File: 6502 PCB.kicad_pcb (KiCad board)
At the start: 2 copper layers, 99.1 x 83.8 mm, 21 parts, among them J1 power_source, J17 Conn_01x16_Pin, J2 Conn_01x02_Pin, SW1 RESET, U1 W65C02S, U2 28C256, U3 62256, U4 W65C22, U5 74HC00, X1 1MHz

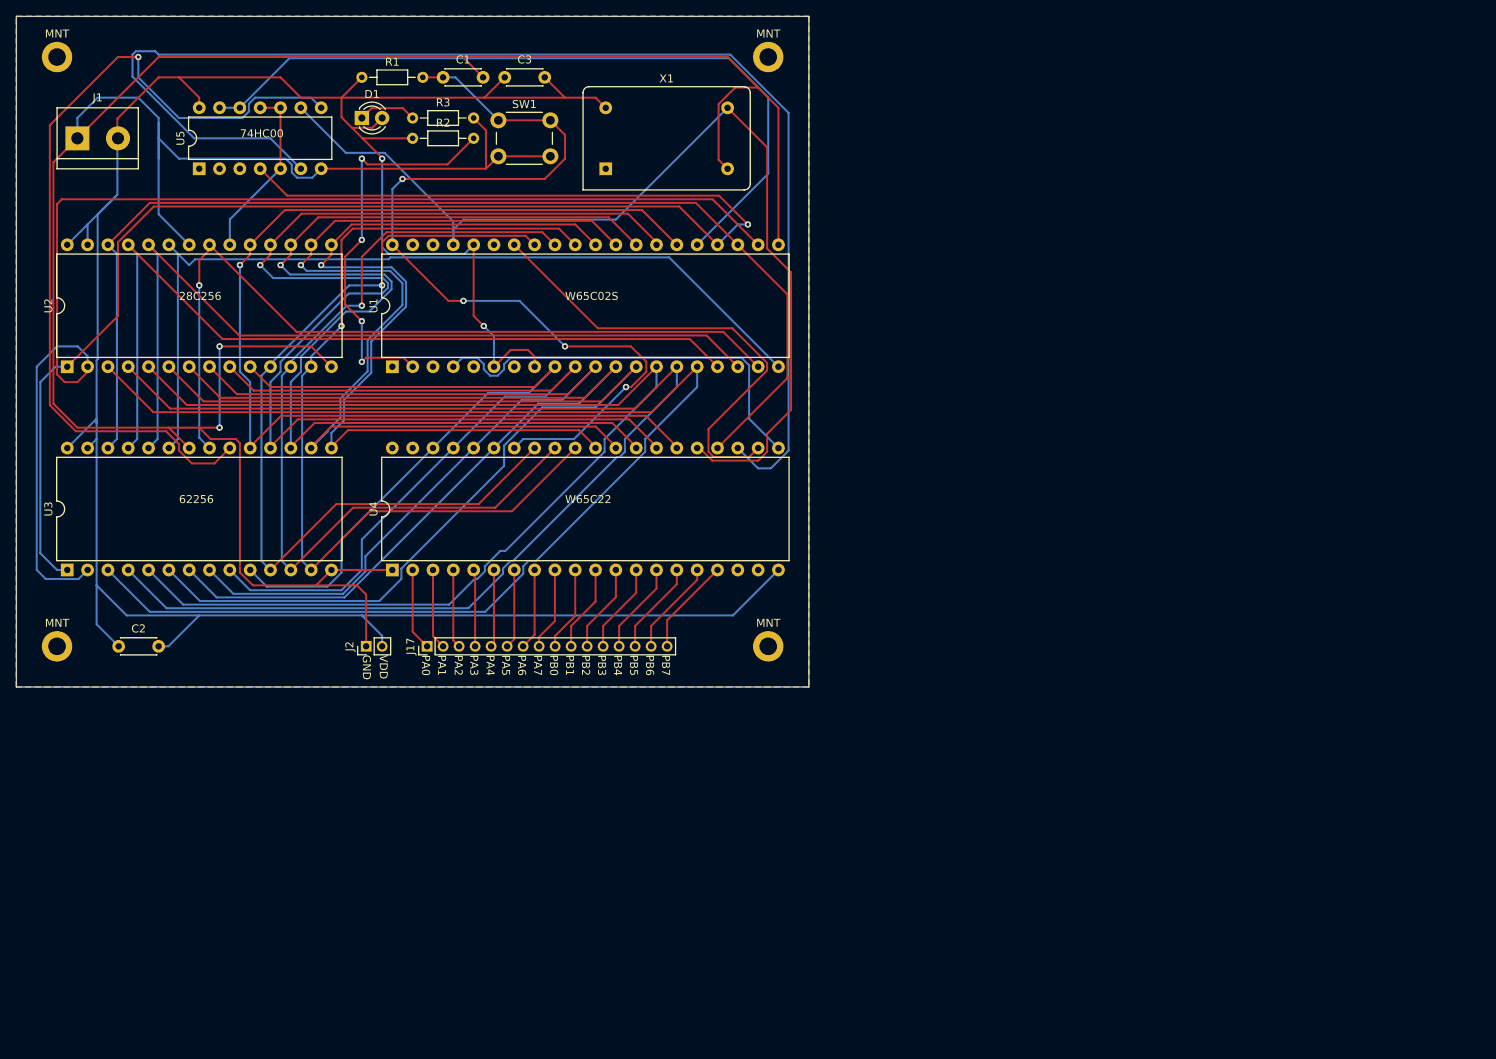
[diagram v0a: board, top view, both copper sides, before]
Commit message: aaaa
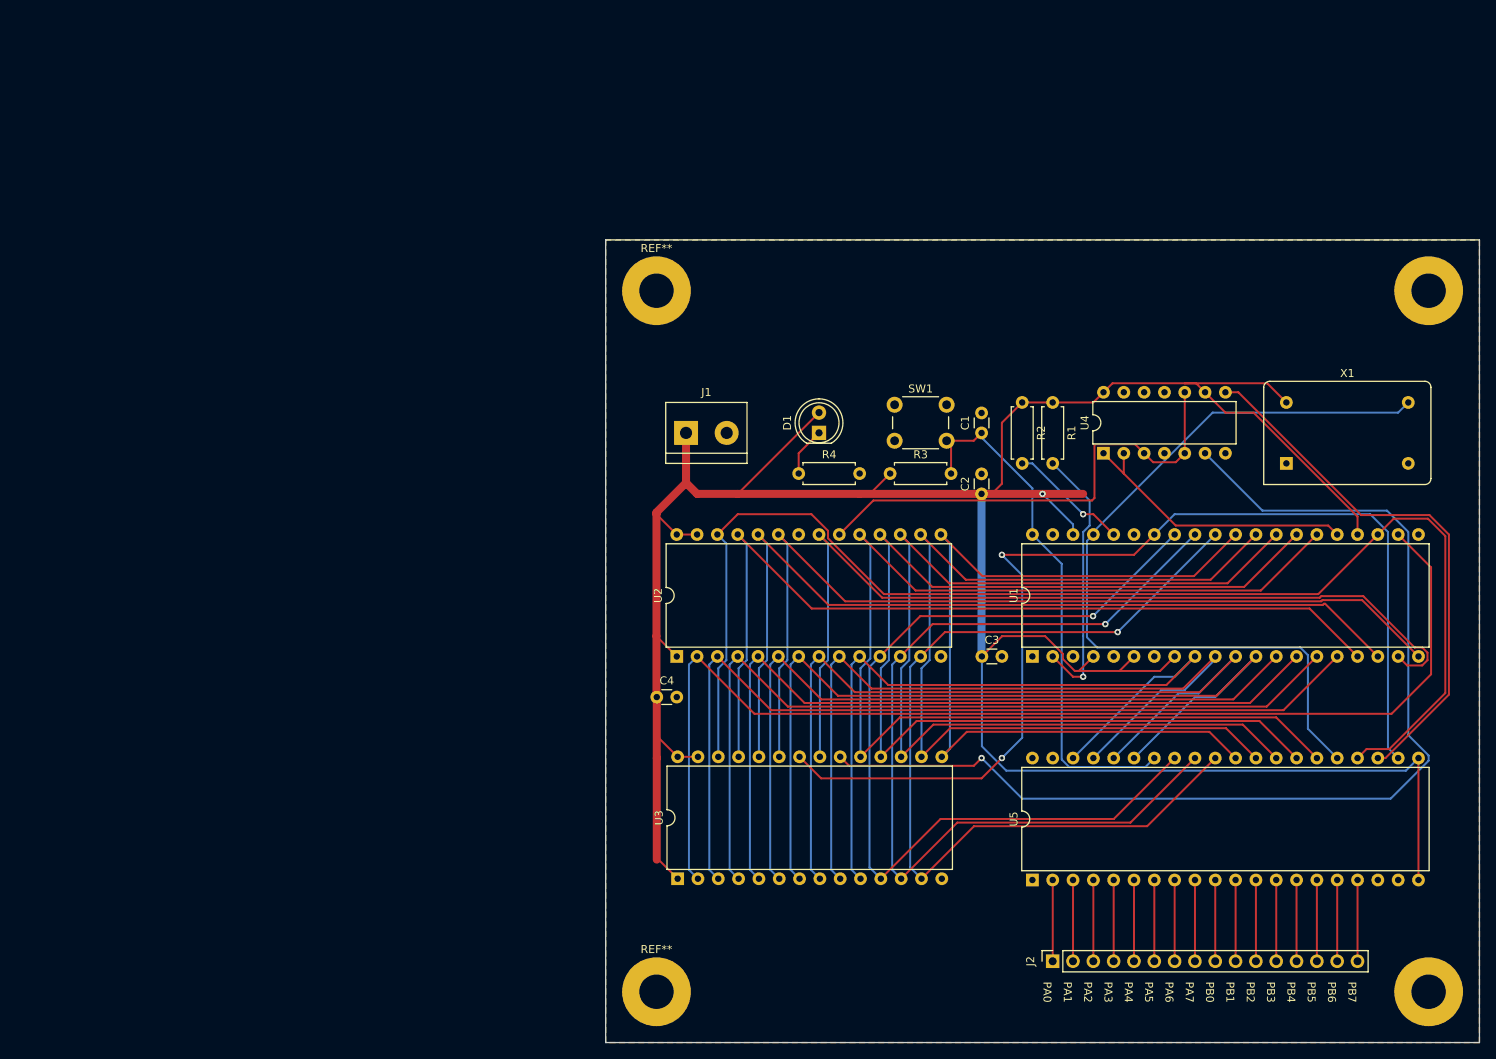
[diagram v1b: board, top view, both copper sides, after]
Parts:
- removed J17: Conn_01x16_Pin, Connector_PinHeader_2.00mm:PinHeader_1x16_P2.00mm_Vertical
- removed MNT (x4): MountingHole_2.2mm_M2_DIN965_Pad, MountingHole:MountingHole_2.2mm_M2_DIN965_Pad
- added ?: , , F.Cu at (189.2, 134.6)
- added ?: , , F.Cu at (189.2, 47.0)
- added C4: 01.uF, Capacitor_THT:C_Disc_D3.0mm_W1.6mm_P2.50mm, F.Cu at (92.7, 97.8)
- added R4: 3.3k, Resistor_THT:R_Axial_DIN0207_L6.3mm_D2.5mm_P7.62mm_Horizontal, F.Cu at (110.5, 69.8)
- added REF**: MountingHole_4.3mm_M4_Pad, MountingHole:MountingHole_4.3mm_M4_Pad, F.Cu at (92.7, 47.0)
- added REF**: MountingHole_4.3mm_M4_Pad, MountingHole:MountingHole_4.3mm_M4_Pad, F.Cu at (92.7, 134.6)
- C1: value 0.1uf -> 0.1uF; footprint Capacitor_THT:C_Disc_D4.3mm_W1.9mm_P5.00mm -> Capacitor_THT:C_Disc_D3.0mm_W1.6mm_P2.50mm
- C2, C3: value 0.1uf -> 01.uF; footprint Capacitor_THT:C_Disc_D4.3mm_W1.9mm_P5.00mm -> Capacitor_THT:C_Disc_D3.0mm_W1.6mm_P2.50mm
- D1: footprint LED_THT:LED_D3.0mm -> LED_THT:LED_D5.0mm
- J1: value power_source -> Screw_Terminal_01x02
- J2: value Conn_01x02_Pin -> Conn_01x16_Pin; footprint Connector_PinHeader_2.00mm:PinHeader_1x02_P2.00mm_Vertical -> Connector_PinSocket_2.54mm:PinSocket_1x16_P2.54mm_Vertical
- R1, R2, R3: value 1K -> 1k; footprint Resistor_THT:R_Axial_DIN0204_L3.6mm_D1.6mm_P7.62mm_Horizontal -> Resistor_THT:R_Axial_DIN0207_L6.3mm_D2.5mm_P7.62mm_Horizontal
- U3: value 62256 -> HM62256BLP
- U4: value W65C22 -> 74HC00; footprint Package_DIP:DIP-40_W15.24mm -> Package_DIP:DIP-14_W7.62mm
- U5: value 74HC00 -> WD65C22; footprint Package_DIP:DIP-14_W7.62mm -> Package_DIP:DIP-40_W15.24mm
- moved U5 136.9 mm to (139.7, 120.7)
- moved C2 109.5 mm to (133.3, 72.4), turned to 90 degrees
- moved R1 95.4 mm to (142.2, 61.0), turned to -90 degrees
- moved J2 94.4 mm to (142.2, 130.8)
- moved C3 93.8 mm to (133.4, 92.7)
- moved X1 92.7 mm to (171.4, 68.6)
- moved U4 90.1 mm to (148.6, 67.3)
- moved U1 87.8 mm to (139.7, 92.7)
- moved U3 85.5 mm to (95.4, 120.5)
- moved J1 84.5 mm to (96.4, 64.8)
- moved U2 84.4 mm to (95.2, 92.7)
- moved R2 83.0 mm to (138.4, 61.0), turned to -90 degrees
- moved C1 80.7 mm to (133.3, 64.8), turned to 90 degrees
- moved R3 74.4 mm to (121.9, 69.8)
- moved D1 69.4 mm to (113.0, 64.8), turned to 90 degrees
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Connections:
- net /a10 renamed /A10
- net /a11 renamed /A11
- net /a12 renamed /A12
- net /a4 renamed /A4
- net /a5 renamed /A5
- net /a6 renamed /A6
- net /a7 renamed /A7
- net /a8 renamed /A8
- net /a9 renamed /A9
- C1 pad 1: Net-(U1-~{RES}) -> /~{RES}
- C1 pad 2: /GND -> GND
- C2 pad 1: /VDD -> +5V
- C2 pad 2: /VDD -> GND
- C3 pad 1: /VDD -> +5V
- C3 pad 2: /VDD -> GND
- D1 pad 2: /VDD -> +5V
- J1 pad 1: /GND -> +5V
- J1 pad 2: /VDD -> GND
- J2 pad 1: /GND -> Net-(J2-Pin_1)
- J2 pad 2: /VDD -> Net-(J2-Pin_2)
- R1 pad 1: /VDD -> +5V
- R1 pad 2: Net-(U1-~{RES}) -> Net-(U1-RDY)
- R2 pad 1: /VDD -> +5V
- R2 pad 2: Net-(U1-RDY) -> Net-(U1-BE)
- R3 pad 1: Net-(D1-K) -> +5V
- R3 pad 2: /GND -> /~{RES}
- SW1 pad 1: Net-(U1-~{RES}) -> GND
- SW1 pad 2: /GND -> /~{RES}
- U1 pad 10: /a1 -> /A1
- U1 pad 11: /a2 -> /A2
- U1 pad 12: /a3 -> /A3
- U1 pad 21: /GND -> GND
- U1 pad 23: /a13 -> /A13
- U1 pad 24: /a14 -> +5V
- U1 pad 25: /a15 -> /A15
- U1 pad 26: /d7 -> /D7
- U1 pad 27: /d6 -> /D6
- U1 pad 28: /d5 -> /D5
- U1 pad 29: /d4 -> /D4
- U1 pad 30: /d3 -> /D3
- U1 pad 31: /d2 -> /D2
- U1 pad 32: /d1 -> /D1
- U1 pad 33: /d0 -> /D0
- U1 pad 34: Net-(U1-R/~{W}) -> /~{RAMWE}
- U1 pad 36: /VDD -> Net-(U1-BE)
- U1 pad 37: Net-(U1-ϕ0) -> /PHI2
- U1 pad 38: unconnected-(U1-~{SO}-Pad38) -> +5V
- U1 pad 4: Net-(U1-~{IRQ}) -> +5V
- U1 pad 40: Net-(U1-~{RES}) -> /~{RES}
- U1 pad 6: /VDD -> +5V
- U1 pad 8: /VDD -> +5V
- U1 pad 9: /a0 -> /A0
- U2 pad 1: /a14 -> +5V
- U2 pad 10: /a0 -> /A0
- U2 pad 11: /d0 -> /D0
- U2 pad 12: /d1 -> /D1
- U2 pad 13: /d2 -> /D2
- U2 pad 14: /GND -> GND
- U2 pad 15: /d3 -> /D3
- U2 pad 16: /d4 -> /D4
- U2 pad 17: /d5 -> /D5
- U2 pad 18: /d6 -> /D6
- U2 pad 19: /d7 -> /D7
- U2 pad 20: Net-(U2-~{CS}) -> +5V
- U2 pad 22: /GND -> GND
- U2 pad 26: /a13 -> /A13
- U2 pad 27: /VDD -> +5V
- U2 pad 28: /VDD -> +5V
- U2 pad 7: /a3 -> /A3
- U2 pad 8: /a2 -> /A2
- U2 pad 9: /a1 -> /A1
- U3 pad 1: /a14 -> +5V
- U3 pad 10: /a0 -> /A0
- U3 pad 11: /d0 -> /D0
- U3 pad 12: /d1 -> /D1
- U3 pad 13: /d2 -> /D2
- U3 pad 14: /GND -> GND
- U3 pad 15: /d3 -> /D3
- U3 pad 16: /d4 -> /D4
- U3 pad 17: /d5 -> /D5
- U3 pad 18: /d6 -> /D6
- U3 pad 19: /d7 -> /D7
- U3 pad 20: Net-(U3-~{CS}) -> /~{RAMCS}
- U3 pad 22: /GND -> /~{RAMWE}
- U3 pad 26: /a13 -> /A13
- U3 pad 27: /VDD -> +5V
- U3 pad 28: /VDD -> +5V
- U3 pad 7: /a3 -> /A3
- U3 pad 8: /a2 -> /A2
- U3 pad 9: /a1 -> /A1
- U4 pad 1: /GND -> /A15
- U4 pad 10: Net-(J17-Pin_9) -> +5V
- U4 pad 11: Net-(J17-Pin_10) -> unconnected-(U4-Pad11)
- U4 pad 12: Net-(J17-Pin_11) -> unconnected-(U4-Pad12)
- U4 pad 13: Net-(J17-Pin_12) -> unconnected-(U4-Pad13)
- U4 pad 14: Net-(J17-Pin_13) -> +5V
- U4 pad 2: Net-(J17-Pin_1) -> /A15
- U4 pad 3: Net-(J17-Pin_2) -> +5V
- U4 pad 4: Net-(J17-Pin_3) -> /PHI2
- U4 pad 5: Net-(J17-Pin_4) -> +5V
- U4 pad 6: Net-(J17-Pin_5) -> /~{RAMCS}
- U4 pad 7: Net-(J17-Pin_6) -> GND
- U4 pad 8: Net-(J17-Pin_7) -> /~{CS2VIA}
- U4 pad 9: Net-(J17-Pin_8) -> +5V
- U5 pad 1: (no net) -> GND
- U5 pad 10: Net-(U2-~{CS}) -> Net-(J2-Pin_9)
- U5 pad 11: Net-(U2-~{CS}) -> Net-(J2-Pin_10)
- U5 pad 12: /a15 -> Net-(J2-Pin_11)
- U5 pad 13: /a15 -> Net-(J2-Pin_12)
- U5 pad 14: (no net) -> Net-(J2-Pin_13)
- U5 pad 2: (no net) -> Net-(J2-Pin_1)
- U5 pad 3: (no net) -> Net-(J2-Pin_2)
- U5 pad 4: /a14 -> Net-(J2-Pin_3)
- U5 pad 5: Net-(U2-~{CS}) -> Net-(J2-Pin_4)
- U5 pad 6: Net-(U4-~{CS2}) -> Net-(J2-Pin_5)
- U5 pad 7: (no net) -> Net-(J2-Pin_6)
- U5 pad 8: Net-(U3-~{CS}) -> Net-(J2-Pin_7)
- U5 pad 9: Net-(U1-ϕ0) -> Net-(J2-Pin_8)
- X1 pad 14: /VDD -> +5V
- X1 pad 7: /GND -> GND
- X1 pad 8: Net-(U1-ϕ0) -> /PHI2
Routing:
- net +5V: track 0.00 -> 434.5 mm, vias 0 -> 1
- net /GND: track 371.9 -> 0.00 mm, vias 2 -> 0
- net /VDD: track 335.2 -> 0.00 mm, vias 2 -> 0
- net /a14: track 195.5 -> 0.00 mm, vias 1 -> 0
- net Net-(U4-~{CS2}): track 164.5 -> 0.00 mm
- net /A13: track 0.00 -> 164.2 mm
- net /D7: track 0.00 -> 153.0 mm
- net /d6: track 151.9 -> 0.00 mm, vias 1 -> 0
- net /D6: track 0.00 -> 141.9 mm
- net /a13: track 141.0 -> 0.00 mm
- net /d7: track 139.9 -> 0.00 mm, vias 1 -> 0
- net /~{RAMCS}: track 0.00 -> 137.6 mm, vias 0 -> 1
- net /d5: track 137.2 -> 0.00 mm, vias 1 -> 0
- net /~{RAMWE}: track 0.00 -> 135.0 mm, vias 0 -> 2
- net /D5: track 0.00 -> 131.0 mm
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- added copper zone on B.Cu, net GND
- added copper zone on F.Cu, net GND
- removed copper zone on B.Cu, net /GND
- removed copper zone on F.Cu, net /GND
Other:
- board size 99.1 x 83.8 mm -> 109.2 x 100.3 mm
- board text added: "Joseph Hanger 6502 2024"
- board text removed: "28C256"
- board text removed: "62256"
- board text removed: "74HC00"
- board text removed: "GND"
- board text removed: "Joseph Hanger 6502 2023"
- board text removed: "VDD"
- board text removed: "W65C02S"
- board text removed: "W65C22"

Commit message: finished PCB Design
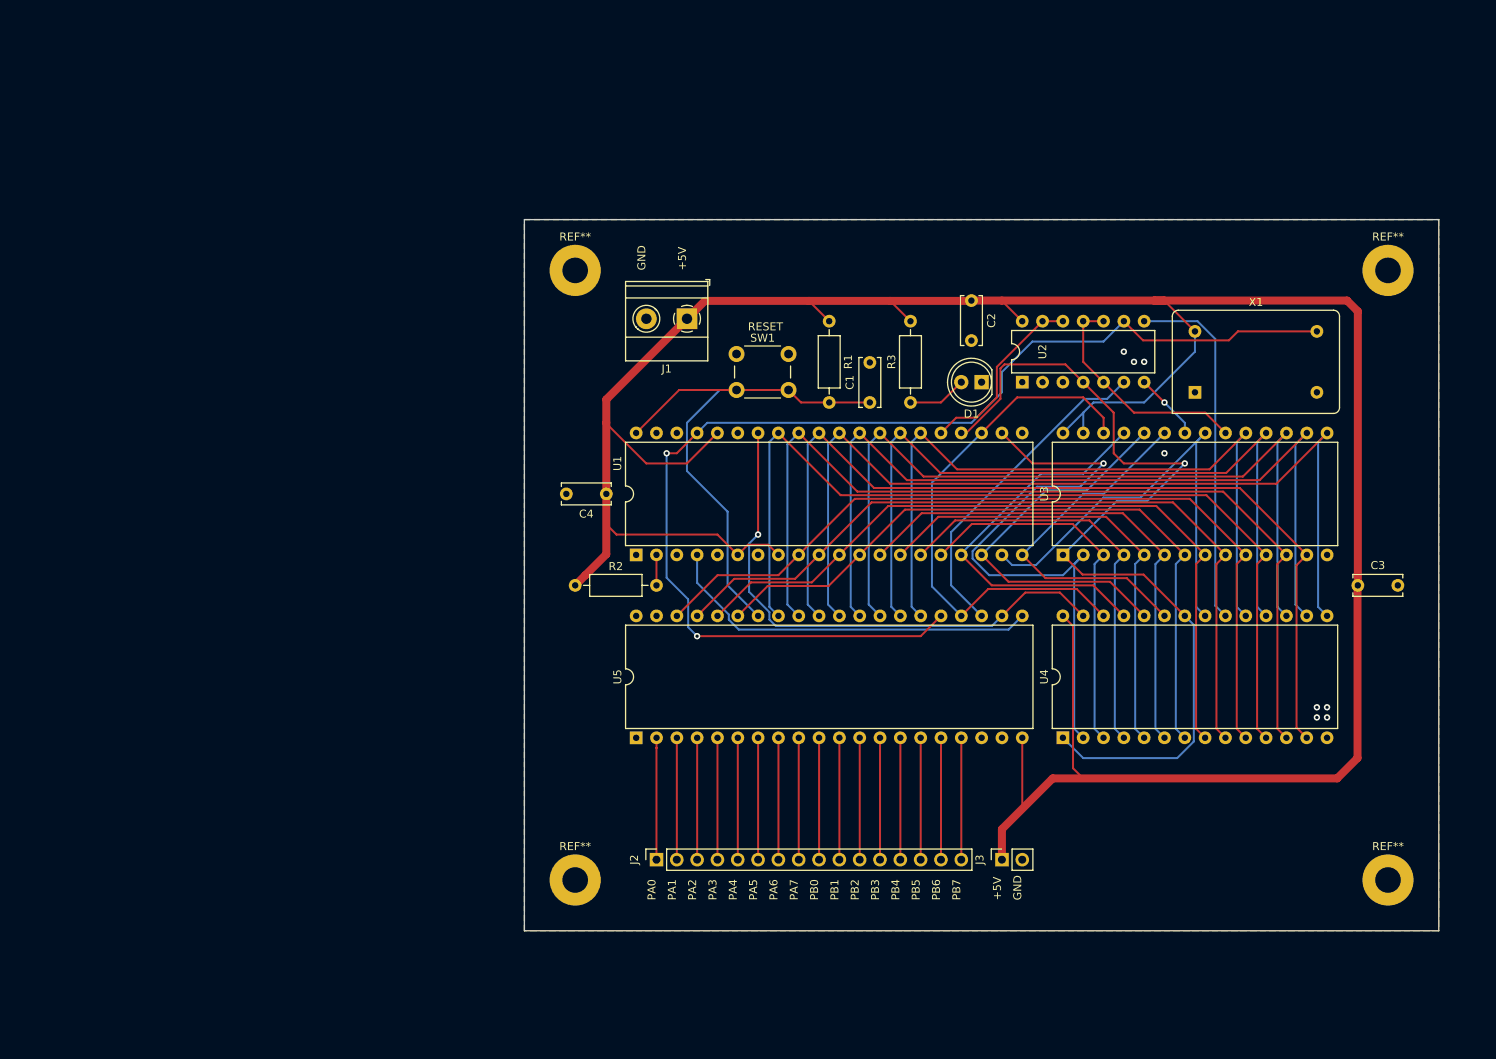
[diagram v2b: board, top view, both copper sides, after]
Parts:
- removed ? (x2): , 
- removed R4: 3.3k, Resistor_THT:R_Axial_DIN0207_L6.3mm_D2.5mm_P7.62mm_Horizontal
- removed the REF** at (92.7, 47.0)
- removed the REF** at (92.7, 134.6)
- added J3: Conn_01x02_Pin, Connector_PinSocket_2.54mm:PinSocket_1x02_P2.54mm_Vertical, F.Cu at (135.9, 118.1)
- added REF**: MountingHole_3.2mm_M3_Pad, MountingHole:MountingHole_3.2mm_M3_Pad, F.Cu at (184.2, 44.5)
- added REF**: MountingHole_3.2mm_M3_Pad, MountingHole:MountingHole_3.2mm_M3_Pad, F.Cu at (82.5, 120.7)
- added REF**: MountingHole_3.2mm_M3_Pad, MountingHole:MountingHole_3.2mm_M3_Pad, F.Cu at (82.5, 44.5)
- added REF**: MountingHole_3.2mm_M3_Pad, MountingHole:MountingHole_3.2mm_M3_Pad, F.Cu at (184.2, 120.7)
- C1: footprint Capacitor_THT:C_Disc_D3.0mm_W1.6mm_P2.50mm -> Capacitor_THT:C_Disc_D6.0mm_W2.5mm_P5.00mm
- C2, C3, C4: value 01.uF -> 0.1uF; footprint Capacitor_THT:C_Disc_D3.0mm_W1.6mm_P2.50mm -> Capacitor_THT:C_Disc_D6.0mm_W2.5mm_P5.00mm
- D1: footprint LED_THT:LED_D5.0mm -> LED_THT:LED_D5.0mm_Clear
- J1: footprint TerminalBlock:TerminalBlock_bornier-2_P5.08mm -> TerminalBlock_Phoenix:TerminalBlock_Phoenix_MKDS-1,5-2-5.08_1x02_P5.08mm_Horizontal
- R1, R2, R3: footprint Resistor_THT:R_Axial_DIN0207_L6.3mm_D2.5mm_P7.62mm_Horizontal -> Resistor_THT:R_Axial_DIN0207_L6.3mm_D2.5mm_P10.16mm_Horizontal
- SW1: footprint Button_Switch_THT:SW_PUSH_6mm -> Button_Switch_THT:SW_PUSH_6mm_H5mm
- U2: value 28C256 -> 74HC00; footprint Package_DIP:DIP-28_W15.24mm -> Package_DIP:DIP-14_W7.62mm
- U3: value HM62256BLP -> 28C256
- U4: value 74HC00 -> 62256; footprint Package_DIP:DIP-14_W7.62mm -> Package_DIP:DIP-28_W15.24mm
- moved U3 62.9 mm to (143.5, 80.0)
- moved R2 60.4 mm to (82.5, 83.8), turned to 0 degrees
- moved U2 55.1 mm to (138.4, 58.4)
- moved U5 52.6 mm to (90.2, 102.9)
- moved U1 51.1 mm to (90.2, 80.0)
- moved J2 51.1 mm to (92.7, 118.1)
- moved C3 47.8 mm to (180.4, 83.8)
- moved U4 35.9 mm to (143.5, 102.9)
- moved R1 29.7 mm to (114.3, 50.8)
- moved C4 26.2 mm to (86.4, 72.4), turned to 180 degrees
- moved C2 24.2 mm to (132.1, 48.2), turned to -90 degrees
- moved D1 21.3 mm to (133.3, 58.4), turned to 180 degrees
- moved SW1 20.7 mm to (102.7, 54.9)
- moved C1 14.5 mm to (119.4, 61.0)
- moved X1 14.5 mm to (160.0, 59.7)
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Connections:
- C1 pad 1: /~{RES} -> ~{RESET}
- D1 pad 1: Net-(D1-K) -> GND
- D1 pad 2: +5V -> Net-(D1-A)
- R1 pad 2: Net-(U1-RDY) -> ~{RESET}
- R2 pad 2: Net-(U1-BE) -> Net-(U1-RDY)
- R3 pad 1: +5V -> Net-(D1-A)
- R3 pad 2: /~{RES} -> +5V
- SW1 pad 2: /~{RES} -> ~{RESET}
- U1 pad 24: +5V -> /A14
- U1 pad 34: /~{RAMWE} -> R/~{W}
- U1 pad 36: Net-(U1-BE) -> +5V
- U1 pad 37: /PHI2 -> CLK
- U1 pad 38: +5V -> unconnected-(U1-~{SO}-Pad38)
- U1 pad 4: +5V -> ~{IRQ}
- U1 pad 40: /~{RES} -> ~{RESET}
- U2 pad 1: +5V -> (no net)
- U2 pad 10: /A0 -> Net-(U3-~{CS})
- U2 pad 11: /D0 -> Net-(U3-~{CS})
- U2 pad 12: /D1 -> /A15
- U2 pad 13: /D2 -> /A15
- U2 pad 14: GND -> +5V
- U2 pad 2: /A12 -> (no net)
- U2 pad 3: /A7 -> (no net)
- U2 pad 4: /A6 -> /A14
- U2 pad 5: /A5 -> Net-(U3-~{CS})
- U2 pad 6: /A4 -> Net-(U5-~{CS2})
- U2 pad 7: /A3 -> GND
- U2 pad 8: /A2 -> Net-(U4-~{CS})
- U2 pad 9: /A1 -> CLK
- U3 pad 1: +5V -> /A14
- U3 pad 20: /~{RAMCS} -> Net-(U3-~{CS})
- U3 pad 22: /~{RAMWE} -> GND
- U4 pad 1: /A15 -> /A14
- U4 pad 10: +5V -> /A0
- U4 pad 11: unconnected-(U4-Pad11) -> /D0
- U4 pad 12: unconnected-(U4-Pad12) -> /D1
- U4 pad 13: unconnected-(U4-Pad13) -> /D2
- U4 pad 14: +5V -> GND
- U4 pad 2: /A15 -> /A12
- U4 pad 3: +5V -> /A7
- U4 pad 4: /PHI2 -> /A6
- U4 pad 5: +5V -> /A5
- U4 pad 6: /~{RAMCS} -> /A4
- U4 pad 7: GND -> /A3
- U4 pad 8: /~{CS2VIA} -> /A2
- U4 pad 9: +5V -> /A1
- U5 pad 21: +5V -> ~{IRQ}
- U5 pad 22: /~{RAMWE} -> R/~{W}
- U5 pad 23: /~{CS2VIA} -> Net-(U5-~{CS2})
- U5 pad 25: /PHI2 -> CLK
- U5 pad 34: /~{RES} -> ~{RESET}
- X1 pad 8: /PHI2 -> CLK
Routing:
- net CLK: track 0.00 -> 147.0 mm, vias 0 -> 2
- net /~{RAMCS}: track 137.6 -> 0.00 mm, vias 1 -> 0
- net /~{RAMWE}: track 135.0 -> 0.00 mm, vias 2 -> 0
- net /A14: track 0.00 -> 114.6 mm, vias 0 -> 1
- net /PHI2: track 102.5 -> 0.00 mm
- net /A13: track 164.2 -> 67.6 mm
- net +5V: track 434.5 -> 351.2 mm, vias 1 -> 0
- net /A11: track 115.1 -> 45.0 mm
- net /A12: track 144.6 -> 75.7 mm, vias 0 -> 1
- net ~{RESET}: track 0.00 -> 67.8 mm
- net /~{CS2VIA}: track 67.5 -> 0.00 mm
- net R/~{W}: track 0.00 -> 67.3 mm, vias 0 -> 1
- net /~{RES}: track 66.5 -> 0.00 mm
- net /A7: track 111.7 -> 47.3 mm
- net /A9: track 112.6 -> 50.1 mm
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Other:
- board size 109.2 x 100.3 mm -> 114.3 x 88.9 mm
- board text added: "+5V"
- board text added: "GND"
- board text added: "RESET"
- board text removed: "Joseph Hanger 6502 2024"
